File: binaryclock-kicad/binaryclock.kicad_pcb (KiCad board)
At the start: 2 copper layers, 100 x 80 mm, 20 parts, among them J1 Conn_01x03_Pin, J2 AVR-ISP-6, SW1 SW_Push, SW2 SW_Push, SW3 SW_Push, U1 ATmega48-20P, Y1 Crystal

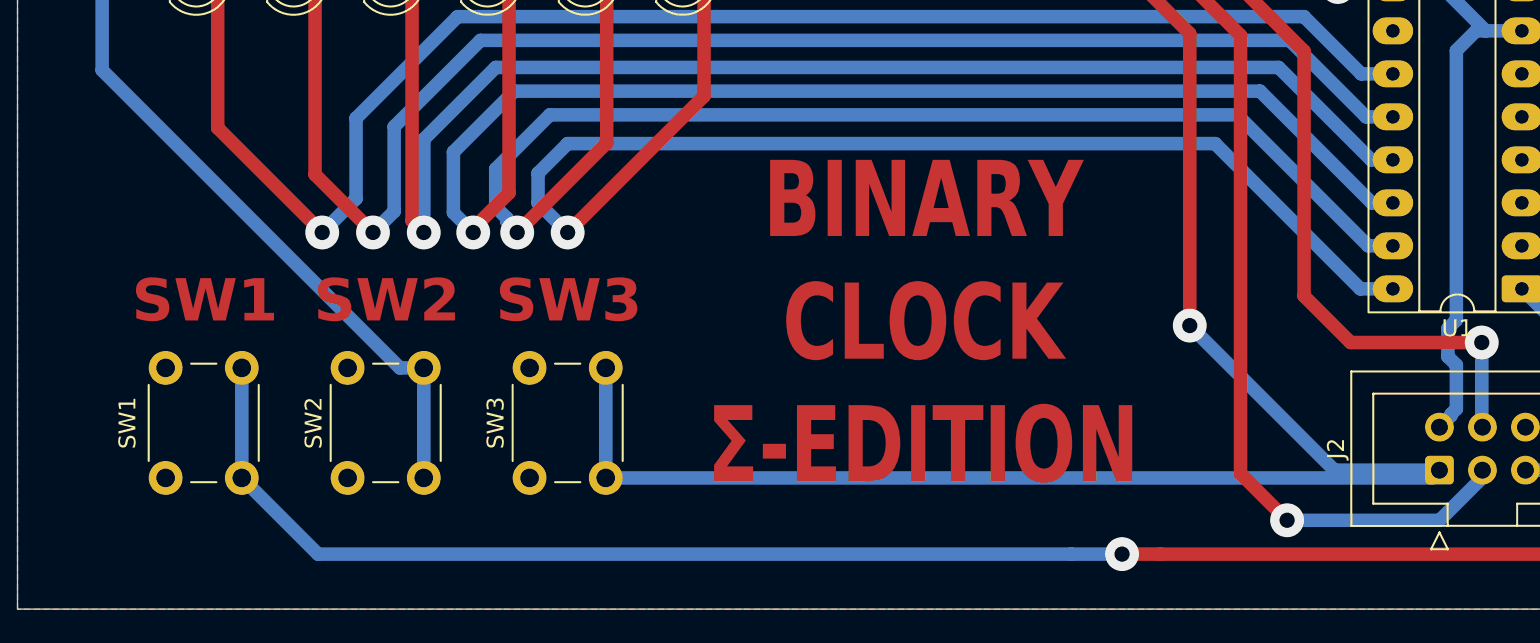
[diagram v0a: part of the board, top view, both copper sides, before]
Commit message: finished pcb
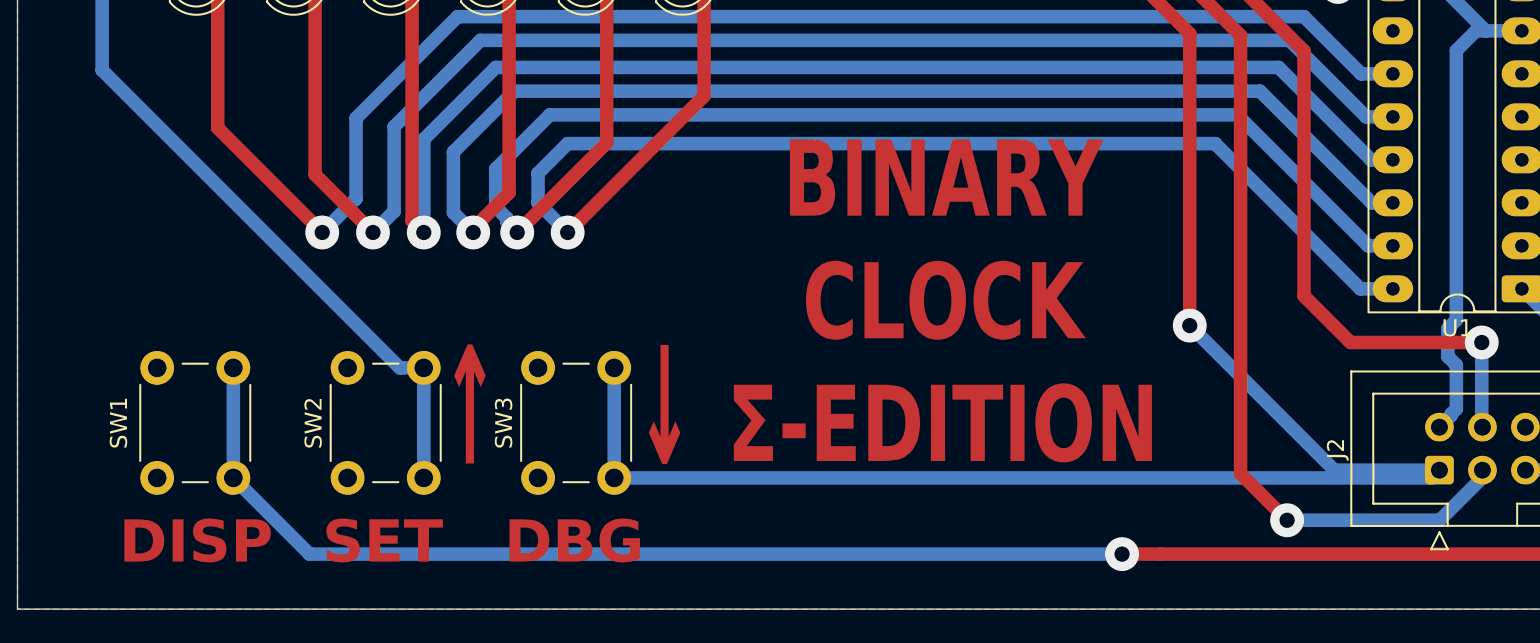
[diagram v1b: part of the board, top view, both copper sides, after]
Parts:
- moved SW1 0.50 mm to (63.2, 112.2)
- moved SW3 0.50 mm to (85.8, 112.2)
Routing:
- net /MISO/PCINT4: track 114.9 -> 114.4 mm
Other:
- board text added: "DBG"
- board text added: "DISP"
- board text added: "SET"
- board text added: "↑"
- board text added: "↓"
- board text removed: "SW1"
- board text removed: "SW2"
- board text removed: "SW3"
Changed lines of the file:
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@@
 		(tenting front back)
 		(pcbplotparams
-			(layerselection 0x00000000_00000000_55555555_57555555)
+			(layerselection 0x00000000_00000000_55555555_55555555)
 			(plot_on_all_layers_selection 0x00000000_00000000_00000000_00000000)
 			(disableapertmacros no)
@@
 			(drillshape 0)
 			(scaleselection 1)
-			(outputdirectory "C:/Users/david/Downloads/")
+			(outputdirectory "../fabrication-outputs/")
 		)
 	)
@@
 	(footprint "Button_Switch_THT:SW_PUSH_6mm"
 		(layer "F.Cu")
-		(at 63.75 112.25 90)
+		(at 63.25 112.25 90)
 		(descr "Generic 6mm SW tactile push button")
 		(tags "tact sw push 6mm")
@@
 	(footprint "Button_Switch_THT:SW_PUSH_6mm"
 		(layer "F.Cu")
-		(at 85.25 112.25 90)
+		(at 85.75 112.25 90)
 		(descr "Generic 6mm SW tactile push button")
 		(tags "tact sw push 6mm")
@@
 		)
 	)
-	(gr_text "SW1"
-		(at 61.75 103.25 0)
+	(gr_text "DISP"
+		(at 61 117.5 0)
 		(layer "F.Cu" knockout)
 		(effects
@@
 		)
 	)
-	(gr_text "SW2"
-		(at 72.5 103.25 0)
+	(gr_text "SET"
+		(at 73 117.5 0)
 		(layer "F.Cu" knockout)
 		(effects
@@
 		)
 	)
-	(gr_text "SW3"
-		(at 83.25 103.25 0)
+	(gr_text "DBG"
+		(at 83.75 117.5 0)
 		(layer "F.Cu" knockout)
 		(effects
@@
 		)
 	)
+	(gr_text "↑"
+		(at 80 112.25 0)
+		(layer "F.Cu" knockout)
+		(effects
+			(font
+				(size 7 3)
+				(thickness 0.6)
+				(bold yes)
+			)
+			(justify left bottom)
+		)
+	)
 	(gr_text "MINUTES"
 		(at 62.75 79.5 0)
@@
 		)
 	)
+	(gr_text "↓"
+		(at 91.5 112.25 0)
+		(layer "F.Cu" knockout)
+		(effects
+			(font
+				(size 7 3)
+				(thickness 0.6)
+				(bold yes)
+			)
+			(justify left bottom)
+		)
+	)
 	(gr_text "BINARY\nCLOCK\nΣ-EDITION"
-		(at 108.5 113 0)
+		(at 109.666661 111.796146 0)
 		(layer "F.Cu" knockout)
 		(effects
@@
 	)
 	(segment
-		(start 132.79 111.79)
+		(start 138.54 112.25)
 		(end 139 111.79)
 		(width 0.8)
@@
 	)
 	(segment
-		(start 89.75 112.25)
-		(end 138.54 112.25)
-		(width 0.8)
-		(layer "B.Cu")
-		(net 21)
-	)
-	(segment
-		(start 124.25 78)
-		(end 126.57 75.68)
+		(start 132.79 111.79)
+		(end 139 111.79)
 		(width 0.8)
 		(layer "B.Cu")
@@
 	)
 	(segment
-		(start 89.75 105.75)
-		(end 89.75 112.25)
+		(start 90.25 105.75)
+		(end 90.25 112.25)
 		(width 0.8)
 		(layer "B.Cu")
@@
 	)
 	(segment
-		(start 138.54 112.25)
-		(end 139 111.79)
+		(start 124.25 78)
+		(end 126.57 75.68)
 		(width 0.8)
 		(layer "B.Cu")
@@
 	)
 	(segment
+		(start 90.25 112.25)
+		(end 138.54 112.25)
+		(width 0.8)
+		(layer "B.Cu")
+		(net 21)
+	)
+	(segment
 		(start 150.499 116.751)
 		(end 152 115.25)
@@
 	)
 	(segment
-		(start 68.25 105.75)
-		(end 68.25 112.25)
-		(width 0.8)
-		(layer "B.Cu")
-		(net 22)
-	)
-	(segment
-		(start 72.751 116.751)
-		(end 68.25 112.25)
-		(width 0.8)
-		(layer "B.Cu")
-		(net 22)
-	)
-	(segment
-		(start 117.249 116.751)
-		(end 72.751 116.751)
+		(start 67.75 112.25)
+		(end 72.25 116.75)
 		(width 0.8)
 		(layer "B.Cu")
@@
 	)
 	(segment
-		(start 117.25 116.75)
-		(end 117.249 116.751)
+		(start 72.25 116.75)
+		(end 120.25 116.75)
 		(width 0.8)
 		(layer "B.Cu")
@@
 	)
 	(segment
-		(start 120.25 116.75)
-		(end 117.25 116.75)
+		(start 67.75 105.75)
+		(end 67.75 112.25)
 		(width 0.8)
 		(layer "B.Cu")
